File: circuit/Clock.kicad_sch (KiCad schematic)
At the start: 15 parts, among them U2 Max98357

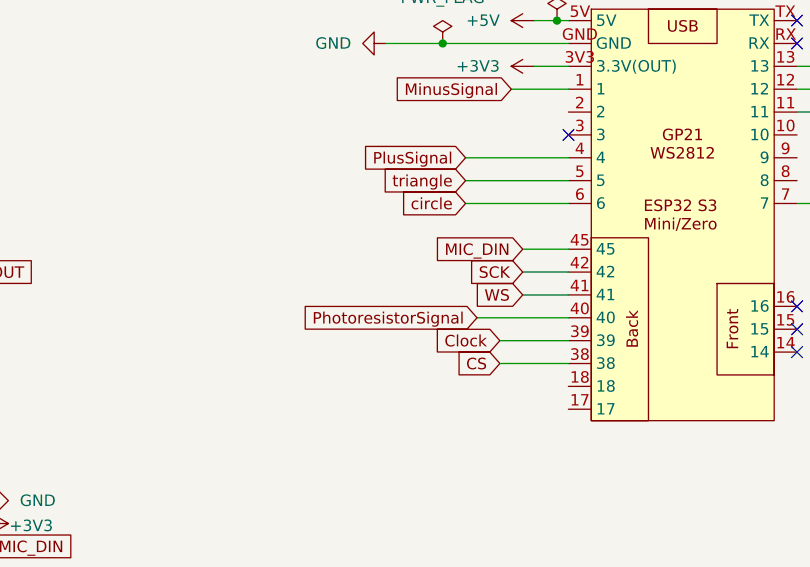
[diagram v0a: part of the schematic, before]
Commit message: more tweaks
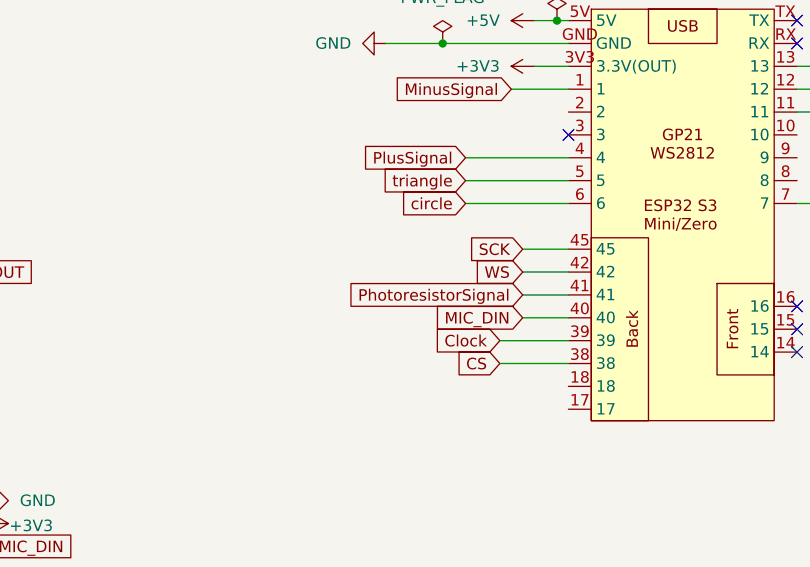
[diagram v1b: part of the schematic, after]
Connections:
- net MIC_DIN: now also ESP32_S1.40; no longer ESP32_S1.45
- net PhotoresistorSignal: now also ESP32_S1.41; no longer ESP32_S1.40
- net SCK: now also ESP32_S1.45; no longer ESP32_S1.42
- net WS: now also ESP32_S1.42; no longer ESP32_S1.41
